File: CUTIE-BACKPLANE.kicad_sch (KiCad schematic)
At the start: 15 parts, among them J7 USB3_A

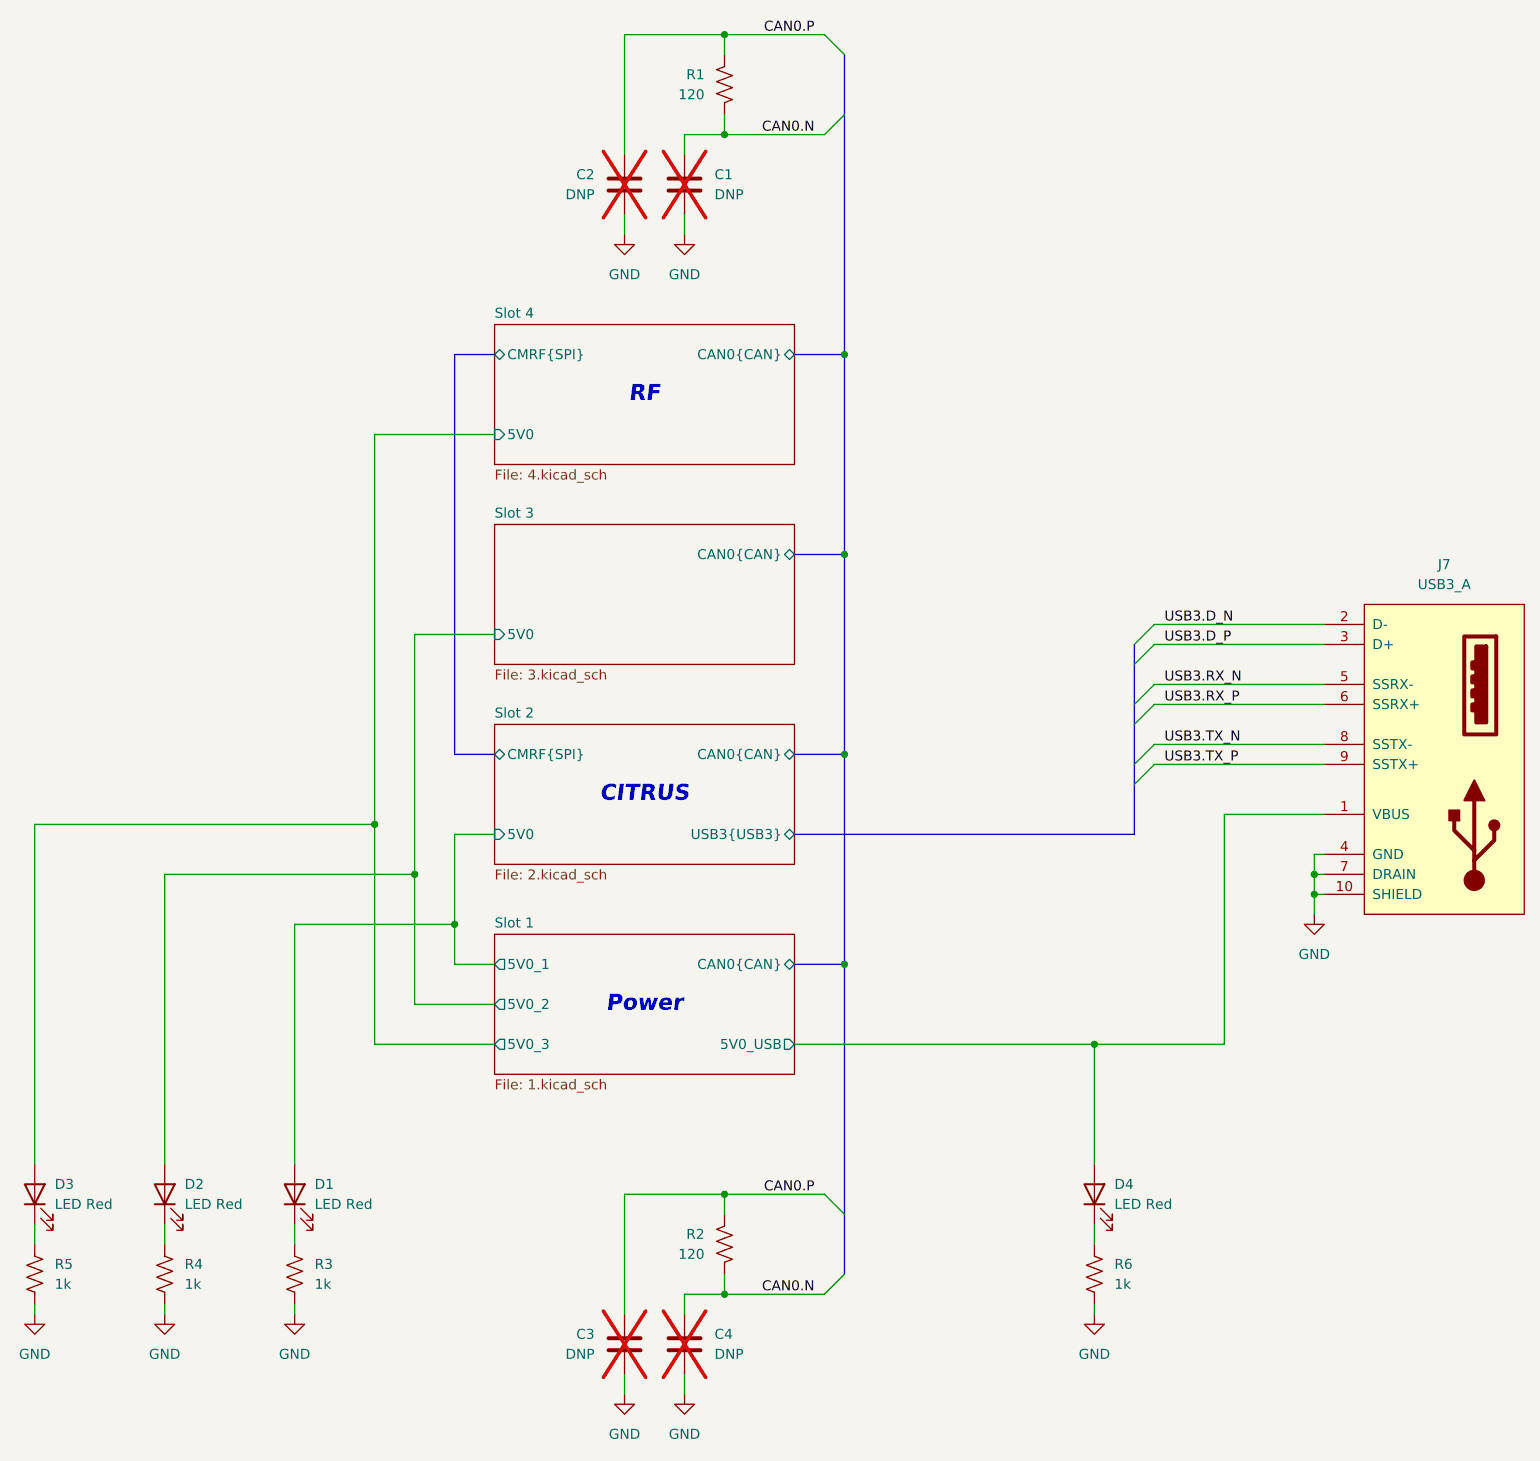
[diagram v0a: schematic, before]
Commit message: added tps and new init layout
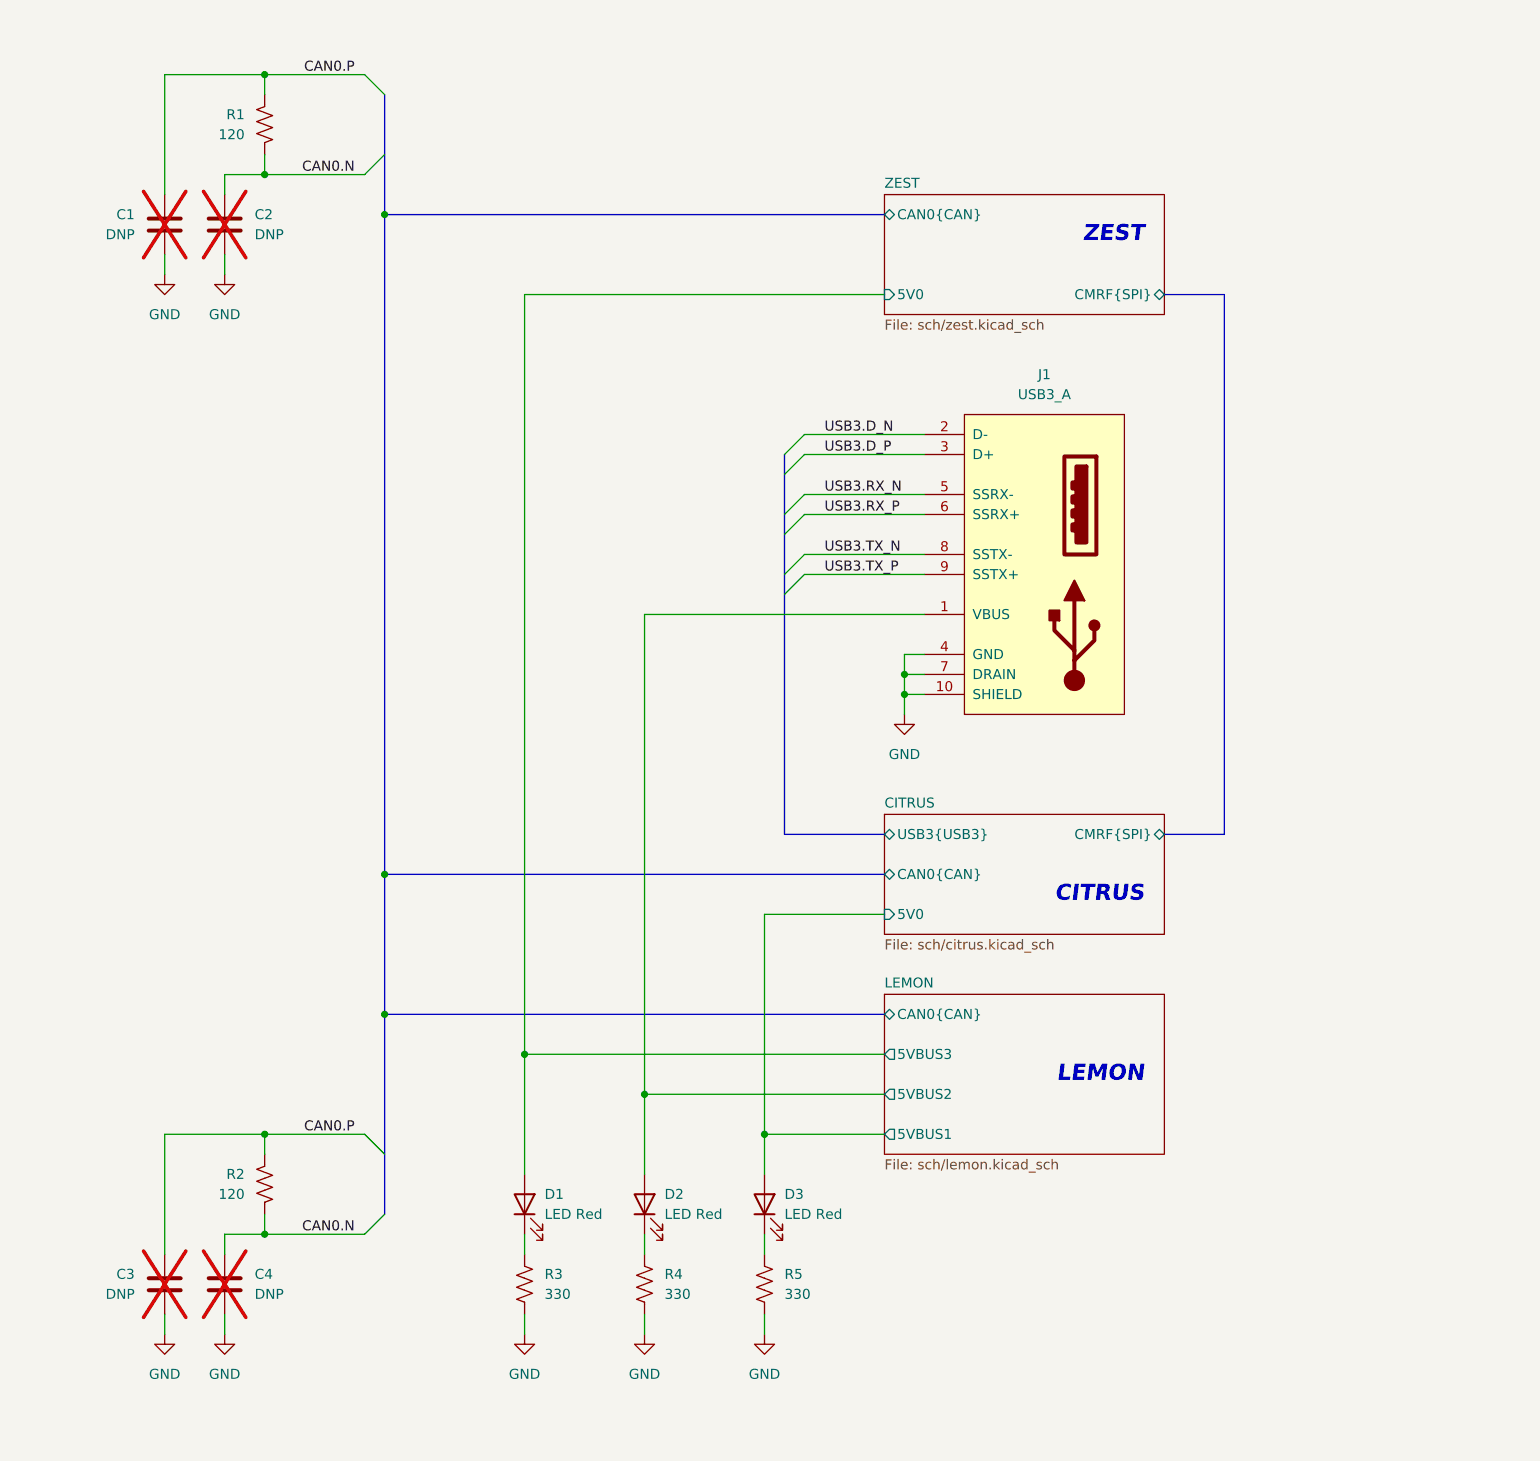
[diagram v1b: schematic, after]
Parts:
- removed D4: LED Red, LED_SMD:LED_0603_1608Metric, symbol library:LED
- removed J7: USB3_A, library:CONN9_08-0003_MOL, symbol Connector:USB3_A
- removed R6: 1k, Resistor_SMD:R_0402_1005Metric, symbol library:R_US
- added J1: USB3_A, library:CONN9_08-0003_MOL, symbol Connector:USB3_A
- R3: renamed from R5; value 1k -> 330
- R4: value 1k -> 330
- R5: renamed from R3; value 1k -> 330
- renumbered D3 to D1, D1 to D3
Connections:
- net CAN0.N: now also C2.2; no longer C1.2
- net CAN0.P: now also C1.2; no longer C2.2
- net GND: now also J1.10 (SHIELD), J1.4 (GND), J1.7 (DRAIN)
- net USB3.D_N: now also J1.2 (D-)
- net USB3.D_P: now also J1.3 (D+)
- net USB3.RX_N: now also J1.5 (SSRX-)
- net USB3.RX_P: now also J1.6 (SSRX+)
- net USB3.TX_N: now also J1.8 (SSTX-)
- net USB3.TX_P: now also J1.9 (SSTX+)
- net LEMON/5V0_1 renamed CITRUS/5V0
- net LEMON/5V0_2 renamed LEMON/5VBUS2
- net LEMON/5VBUS2: now also J1.1 (VBUS)
- net LEMON/5V0_3 renamed LEMON/5VBUS3
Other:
- sheet Slot 1 renamed LEMON
- sheet Slot 2 renamed CITRUS
- sheet Slot 4 renamed ZEST
- removed sheet Slot 3
- sheet CITRUS: file 2.kicad_sch -> sch/citrus.kicad_sch
- sheet LEMON: file 1.kicad_sch -> sch/lemon.kicad_sch
- sheet LEMON ports: added 5VBUS1, 5VBUS2, 5VBUS3; removed 5V0_1, 5V0_2, 5V0_3, 5V0_USB
- sheet ZEST: file 4.kicad_sch -> sch/zest.kicad_sch
- note added: "LEMON"
- note added: "ZEST"
- note removed: "Power"
- note removed: "RF"
- moved on the sheet: D1, D2, D3, R3, R4, R5

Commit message: push for fab
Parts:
- D1, D2, D3: footprint LED_SMD:LED_0603_1608Metric -> LED_SMD:LED_0805_2012Metric; Manufacturer Product Number LTST-S270KRKT -> LTST-C171KRKT
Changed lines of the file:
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@@
-	)
-	(symbol
-		(lib_id "library:LED")
-		(at 119.38 166.37 90)
-		(unit 1)
-		(body_style 1)
-		(exclude_from_sim no)
-		(in_bom yes)
-		(on_board yes)
-		(in_pos_files yes)
-		(dnp no)
-		(property "Reference" "D3"
-			(at 121.92 165.1 90)
-			(show_name no)
-			(do_not_autoplace no)
-			(effects
-				(font
-					(size 1.27 1.27)
-				)
-				(justify right)
-			)
-		)
-		(property "Value" "LED Red"
-			(at 121.92 167.64 90)
-			(show_name no)
-			(do_not_autoplace no)
-			(effects
-				(font
-					(size 1.27 1.27)
-				)
-				(justify right)
-			)
-		)
-		(property "Footprint" "LED_SMD:LED_0603_1608Metric"
-			(at 119.38 166.37 0)
-			(hide yes)
-			(show_name no)
-			(do_not_autoplace no)
-			(effects
-				(font
-					(size 1.27 1.27)
-				)
-			)
-		)
-		(property "Datasheet" "http://optoelectronics.liteon.com/upload/download/DS22-2000-226/LTST-S270KGKT.pdf"
-			(at 119.38 166.37 0)
-			(hide yes)
-			(show_name no)
-			(do_not_autoplace no)
-			(effects
-				(font
-					(size 1.27 1.27)
-				)
-			)
-		)
-		(property "Description" "LED GREEN CLEAR CHIP SMD R/A"
-			(at 119.38 166.37 0)
-			(hide yes)
-			(show_name no)
-			(do_not_autoplace no)
-			(effects
-				(font
-					(size 1.27 1.27)
-				)
-			)
-		)
-		(property "Manufacturer" "Lite-On Inc."
-			(at 119.38 166.37 0)
-			(hide yes)
-			(show_name no)
-			(do_not_autoplace no)
-			(effects
-				(font
-					(size 1.27 1.27)
-				)
-			)
-		)
-		(property "Manufacturer Product Number" "LTST-S270KRKT"
-			(at 119.38 166.37 0)
-			(hide yes)
-			(show_name no)
-			(do_not_autoplace no)
-			(effects
-				(font
-					(size 1.27 1.27)
-				)
-			)
-		)
-		(pin "1"
-		)
-		(pin "2"
-		)
-		(instances
-			(project "CUTIE-BACKPLANE"
-				(path "/db751f7b-eeef-4f9a-a021-6b6484a5d83e"
-					(reference "D3")
-					(unit 1)
-				)
-			)
-		)
 	)
 	(symbol
@@
 	)
 	(symbol
-		(lib_id "library:LED")
-		(at 104.14 166.37 90)
-		(unit 1)
-		(body_style 1)
-		(exclude_from_sim no)
-		(in_bom yes)
-		(on_board yes)
-		(in_pos_files yes)
-		(dnp no)
-		(property "Reference" "D2"
-			(at 106.68 165.1 90)
-			(show_name no)
-			(do_not_autoplace no)
-			(effects
-				(font
-					(size 1.27 1.27)
-				)
-				(justify right)
-			)
-		)
-		(property "Value" "LED Red"
-			(at 106.68 167.64 90)
-			(show_name no)
-			(do_not_autoplace no)
-			(effects
-				(font
-					(size 1.27 1.27)
-				)
-				(justify right)
-			)
-		)
-		(property "Footprint" "LED_SMD:LED_0603_1608Metric"
-			(at 104.14 166.37 0)
-			(hide yes)
-			(show_name no)
-			(do_not_autoplace no)
-			(effects
-				(font
-					(size 1.27 1.27)
-				)
-			)
-		)
-		(property "Datasheet" "http://optoelectronics.liteon.com/upload/download/DS22-2000-226/LTST-S270KGKT.pdf"
-			(at 104.14 166.37 0)
-			(hide yes)
-			(show_name no)
-			(do_not_autoplace no)
-			(effects
-				(font
-					(size 1.27 1.27)
-				)
-			)
-		)
-		(property "Description" "LED GREEN CLEAR CHIP SMD R/A"
-			(at 104.14 166.37 0)
-			(hide yes)
-			(show_name no)
-			(do_not_autoplace no)
-			(effects
-				(font
-					(size 1.27 1.27)
-				)
-			)
-		)
-		(property "Manufacturer" "Lite-On Inc."
-			(at 104.14 166.37 0)
-			(hide yes)
-			(show_name no)
-			(do_not_autoplace no)
-			(effects
-				(font
-					(size 1.27 1.27)
-				)
-			)
-		)
-		(property "Manufacturer Product Number" "LTST-S270KRKT"
-			(at 104.14 166.37 0)
-			(hide yes)
-			(show_name no)
-			(do_not_autoplace no)
-			(effects
-				(font
-					(size 1.27 1.27)
-				)
-			)
-		)
-		(pin "1"
-		)
-		(pin "2"
-		)
-		(instances
-			(project "CUTIE-BACKPLANE"
-				(path "/db751f7b-eeef-4f9a-a021-6b6484a5d83e"
-					(reference "D2")
-					(unit 1)
-				)
-			)
-		)
-	)
-	(symbol
 		(lib_id "Device:C")
 		(at 50.8 176.53 180)
@@
 			)
 		)
-		(property "Footprint" "LED_SMD:LED_0603_1608Metric"
+		(property "Footprint" "LED_SMD:LED_0805_2012Metric"
 			(at 88.9 166.37 0)
 			(hide yes)
@@
 			)
 		)
-		(property "Manufacturer Product Number" "LTST-S270KRKT"
+		(property "Manufacturer Product Number" "LTST-C171KRKT"
 			(at 88.9 166.37 0)
 			(hide yes)
@@
 				(path "/db751f7b-eeef-4f9a-a021-6b6484a5d83e"
 					(reference "D1")
+					(unit 1)
+				)
+			)
+		)
+	)
+	(symbol
+		(lib_id "library:LED")
+		(at 119.38 166.37 90)
+		(unit 1)
+		(body_style 1)
+		(exclude_from_sim no)
+		(in_bom yes)
+		(on_board yes)
+		(in_pos_files yes)
+		(dnp no)
+		(property "Reference" "D3"
+			(at 121.92 165.1 90)
+			(show_name no)
+			(do_not_autoplace no)
+			(effects
+				(font
+					(size 1.27 1.27)
+				)
+				(justify right)
+			)
+		)
+		(property "Value" "LED Red"
+			(at 121.92 167.64 90)
+			(show_name no)
+			(do_not_autoplace no)
+			(effects
+				(font
+					(size 1.27 1.27)
+				)
+				(justify right)
+			)
+		)
+		(property "Footprint" "LED_SMD:LED_0805_2012Metric"
+			(at 119.38 166.37 0)
+			(hide yes)
+			(show_name no)
+			(do_not_autoplace no)
+			(effects
+				(font
+					(size 1.27 1.27)
+				)
+			)
+		)
+		(property "Datasheet" "http://optoelectronics.liteon.com/upload/download/DS22-2000-226/LTST-S270KGKT.pdf"
+			(at 119.38 166.37 0)
+			(hide yes)
+			(show_name no)
+			(do_not_autoplace no)
+			(effects
+				(font
+					(size 1.27 1.27)
+				)
+			)
+		)
+		(property "Description" "LED GREEN CLEAR CHIP SMD R/A"
+			(at 119.38 166.37 0)
+			(hide yes)
+			(show_name no)
+			(do_not_autoplace no)
+			(effects
+				(font
+					(size 1.27 1.27)
+				)
+			)
+		)
+		(property "Manufacturer" "Lite-On Inc."
+			(at 119.38 166.37 0)
+			(hide yes)
+			(show_name no)
+			(do_not_autoplace no)
+			(effects
+				(font
+					(size 1.27 1.27)
+				)
+			)
+		)
+		(property "Manufacturer Product Number" "LTST-C171KRKT"
+			(at 119.38 166.37 0)
+			(hide yes)
+			(show_name no)
+			(do_not_autoplace no)
+			(effects
+				(font
+					(size 1.27 1.27)
+				)
+			)
+		)
+		(pin "1"
+		)
+		(pin "2"
+		)
+		(instances
+			(project "CUTIE-BACKPLANE"
+				(path "/db751f7b-eeef-4f9a-a021-6b6484a5d83e"
+					(reference "D3")
 					(unit 1)
 				)
@@
 					(unit 1)
 				)
+			)
+		)
+	)
+	(symbol
+		(lib_id "library:LED")
+		(at 104.14 166.37 90)
+		(unit 1)
+		(body_style 1)
+		(exclude_from_sim no)
+		(in_bom yes)
+		(on_board yes)
+		(in_pos_files yes)
+		(dnp no)
+		(property "Reference" "D2"
+			(at 106.68 165.1 90)
+			(show_name no)
+			(do_not_autoplace no)
+			(effects
+				(font
+					(size 1.27 1.27)
+				)
+				(justify right)
+			)
+		)
+		(property "Value" "LED Red"
+			(at 106.68 167.64 90)
+			(show_name no)
+			(do_not_autoplace no)
+			(effects
+				(font
+					(size 1.27 1.27)
+				)
+				(justify right)
+			)
+		)
+		(property "Footprint" "LED_SMD:LED_0805_2012Metric"
+			(at 104.14 166.37 0)
+			(hide yes)
+			(show_name no)
+			(do_not_autoplace no)
+			(effects
+				(font
+					(size 1.27 1.27)
+				)
+			)
+		)
+		(property "Datasheet" "http://optoelectronics.liteon.com/upload/download/DS22-2000-226/LTST-S270KGKT.pdf"
+			(at 104.14 166.37 0)
+			(hide yes)
+			(show_name no)
+			(do_not_autoplace no)
+			(effects
+				(font
+					(size 1.27 1.27)
+				)
+			)
+		)
+		(property "Description" "LED GREEN CLEAR CHIP SMD R/A"
+			(at 104.14 166.37 0)
+			(hide yes)
+			(show_name no)
+			(do_not_autoplace no)
+			(effects
+				(font
+					(size 1.27 1.27)
+				)
+			)
+		)
+		(property "Manufacturer" "Lite-On Inc."
+			(at 104.14 166.37 0)
+			(hide yes)
+			(show_name no)
+			(do_not_autoplace no)
+			(effects
+				(font
+					(size 1.27 1.27)
+				)
+			)
+		)
+		(property "Manufacturer Product Number" "LTST-C171KRKT"
+			(at 104.14 166.37 0)
+			(hide yes)
+			(show_name no)
+			(do_not_autoplace no)
+			(effects
+				(font
+					(size 1.27 1.27)
+				)
+			)
+		)
+		(pin "1"
+		)
+		(pin "2"
+		)
+		(instances
+			(project "CUTIE-BACKPLANE"
+				(path "/db751f7b-eeef-4f9a-a021-6b6484a5d83e"
+					(reference "D2")
+					(unit 1)
+				)
